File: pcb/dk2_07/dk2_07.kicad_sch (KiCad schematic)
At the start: 11 parts, among them J1 Trigger_Out_1, J10 Conn_01x03_Pin, J2 Trigger_Out_2, J3 Sync_In, J4 Euro_Out_1, J5 Micro_SD_Card, J6 Trigger_Out_3, J7 Trigger_Out_4, J8 Sync_Out, J9 Euro_Out_2

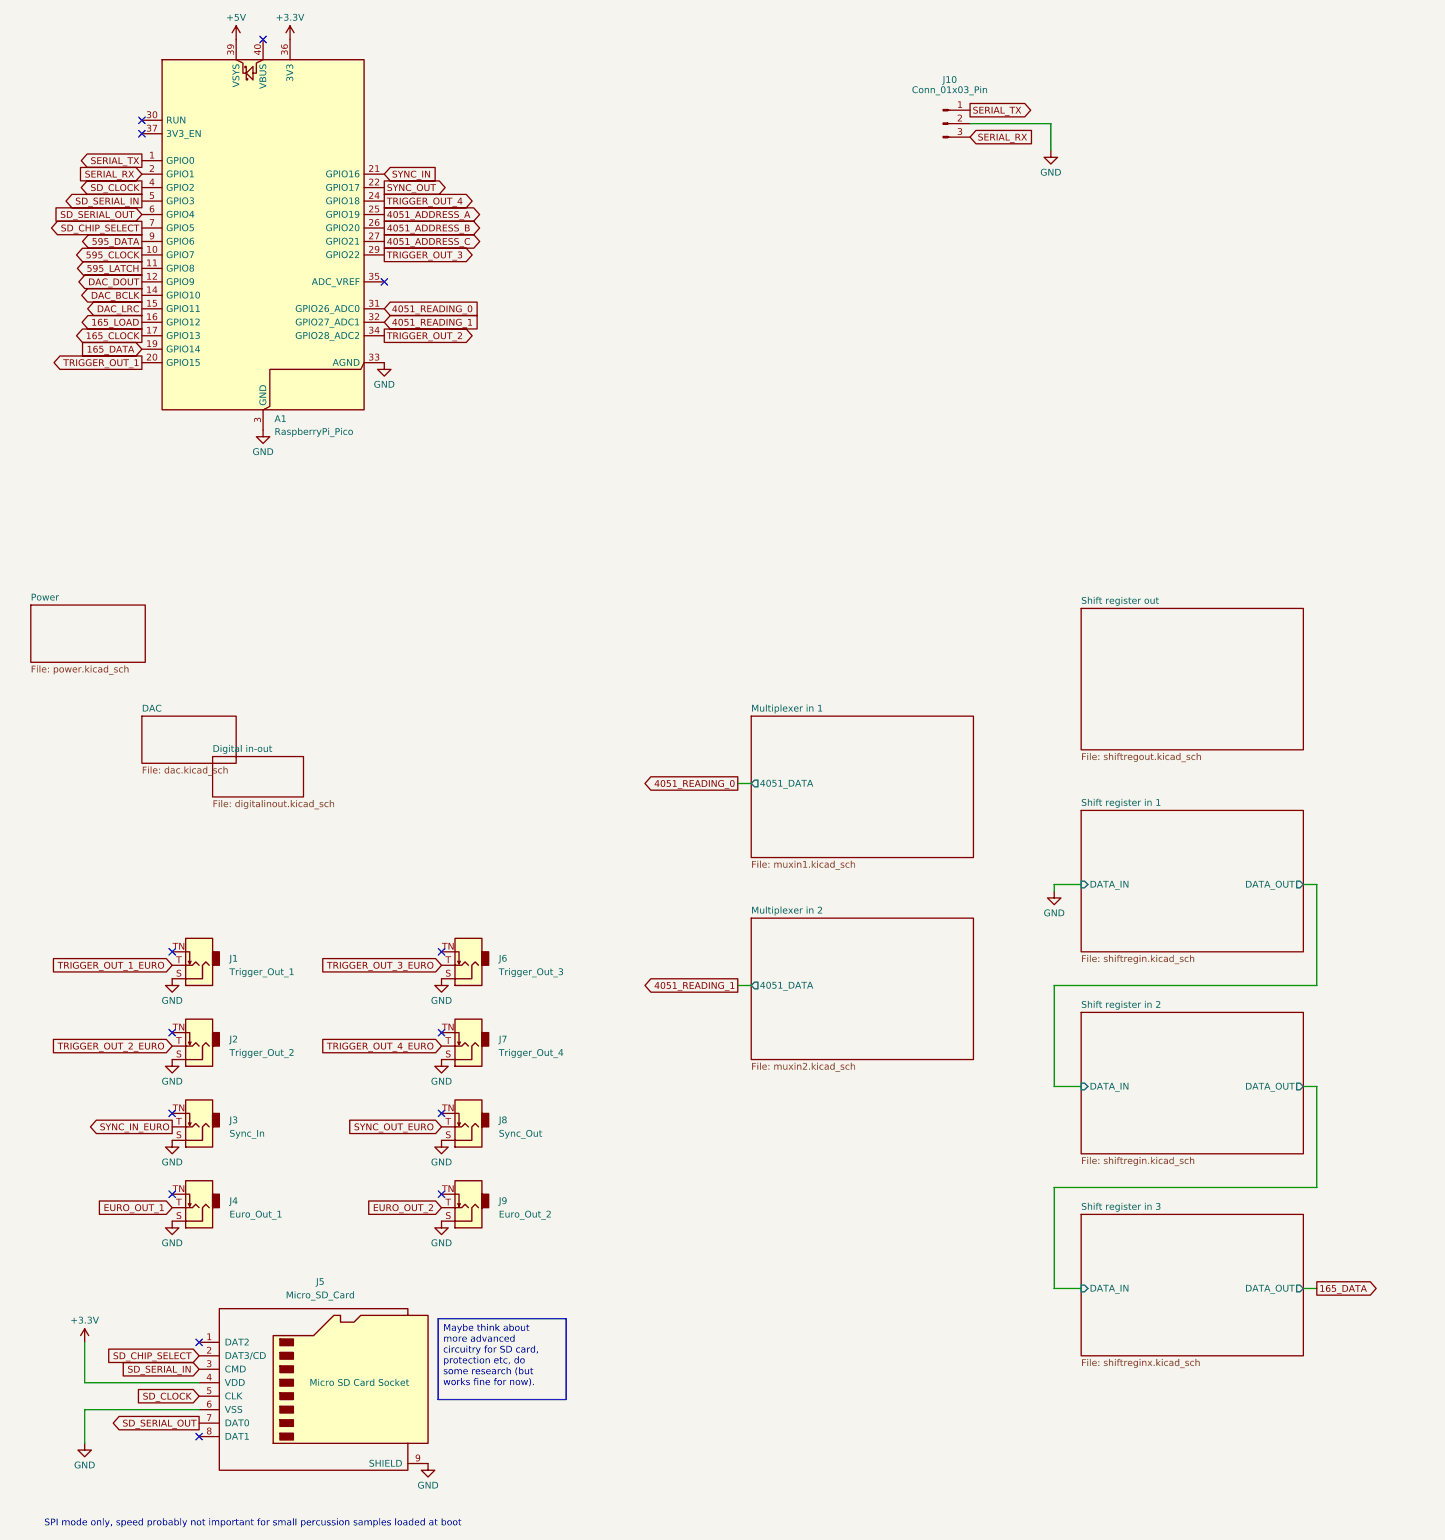
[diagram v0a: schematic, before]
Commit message: pcb v2.07 nearly done
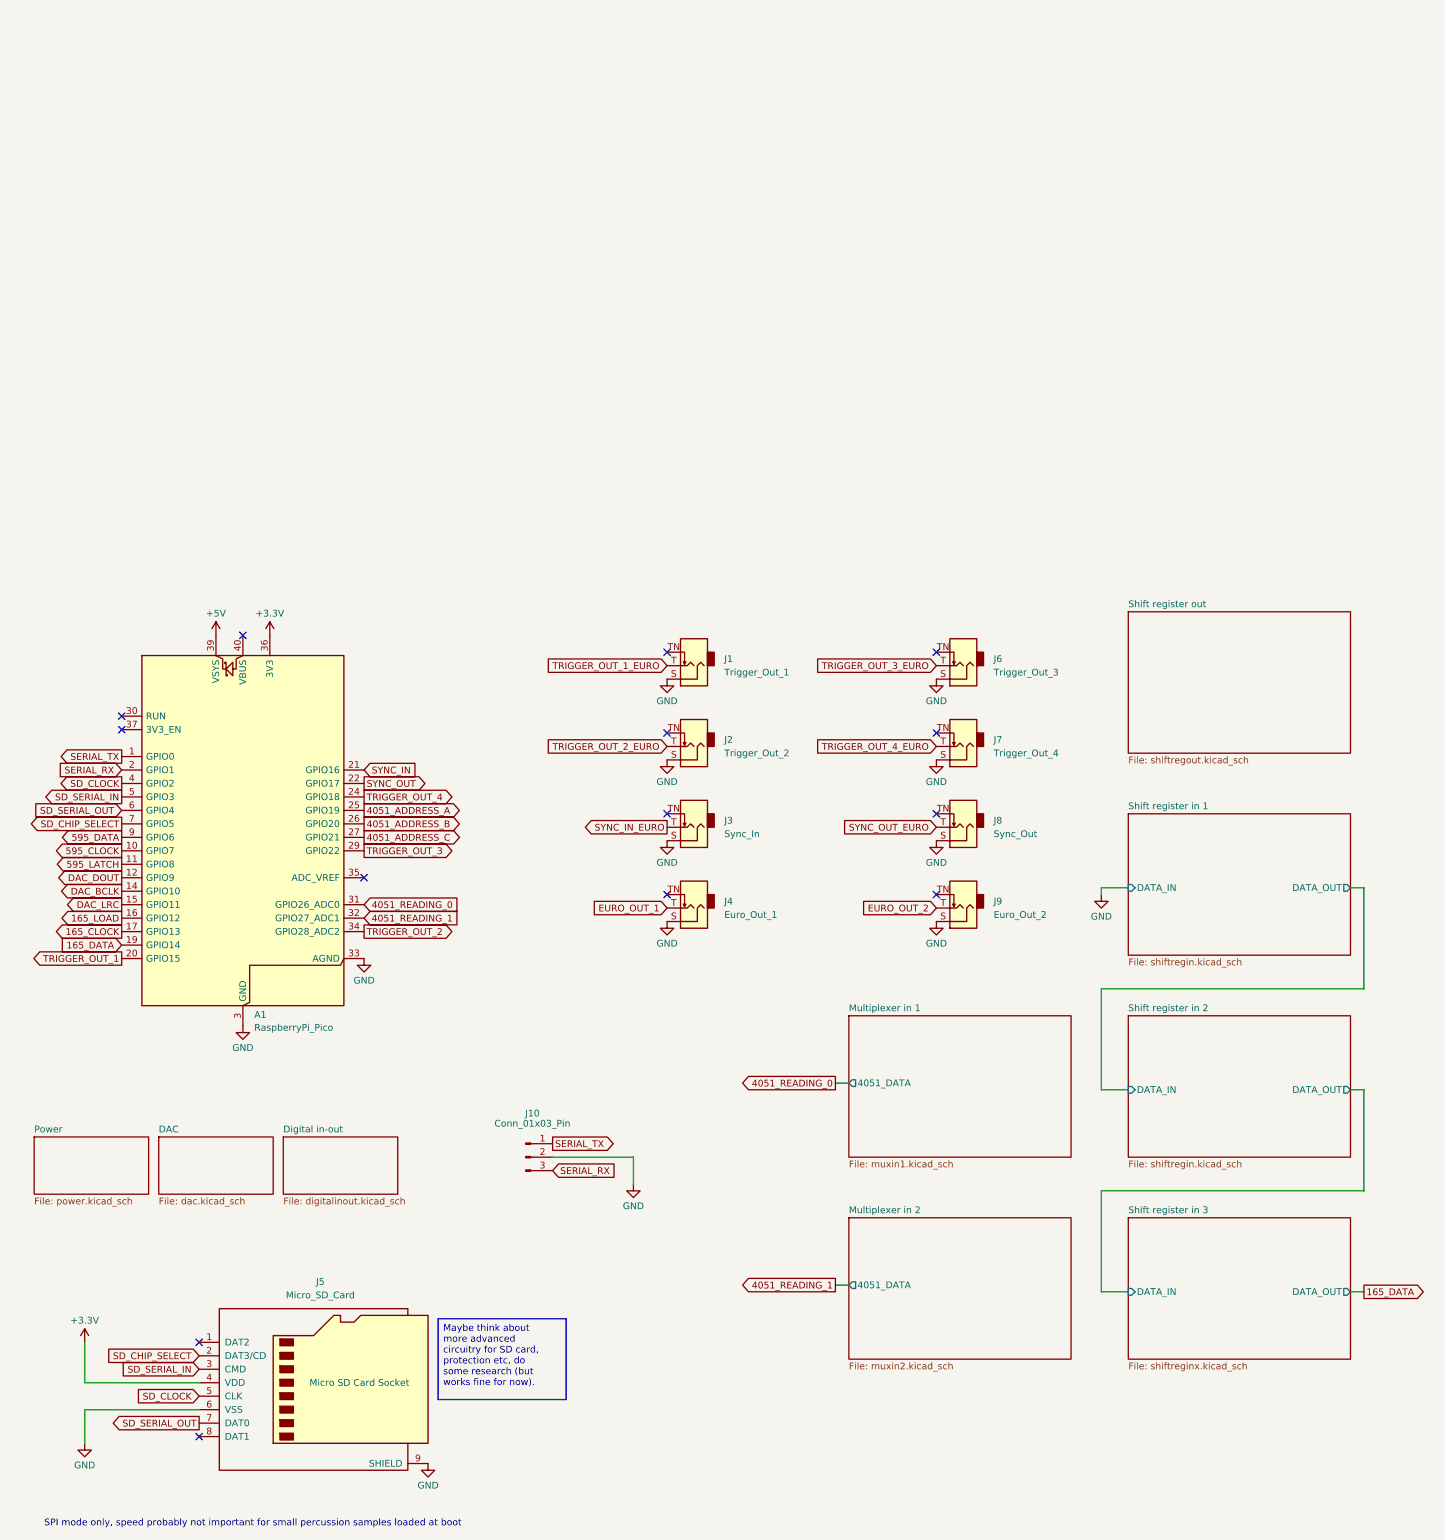
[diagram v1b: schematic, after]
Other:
- moved on the sheet: A1, J1, J10, J2, J3, J4, J6, J7, J8, J9
